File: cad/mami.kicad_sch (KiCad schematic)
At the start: 86 parts, among them SW1 SW_Push, SW10 SW_Push, SW11 SW_Push, SW12 SW_Push, SW13 SW_Push, SW14 SW_Push, SW15 SW_Push, SW16 SW_Push, SW17 SW_Push, SW18 SW_Push, SW19 SW_Push, SW2 SW_Push, SW20 SW_Push, SW21 SW_Push, SW22 SW_Push, SW23 SW_Push, SW24 SW_Push, SW25 SW_Push, SW26 SW_Push, SW27 SW_Push, SW28 SW_Push, SW29 SW_Push, SW3 SW_Push, SW30 SW_Push, SW31 SW_Push, SW32 SW_Push, SW33 SW_Push, SW34 SW_Push, SW35 SW_Push, SW36 SW_Push, SW37 SW_Push, SW38 SW_Push, SW39 SW_Push, SW4 SW_Push, SW40 SW_Push, SW41 SW_Push, SW42 SW_Push, SW43 ResetSW, SW5 SW_Push, SW6 SW_Push, SW7 SW_Push, SW8 SW_Push, SW9 SW_Push, U1 ProMicro

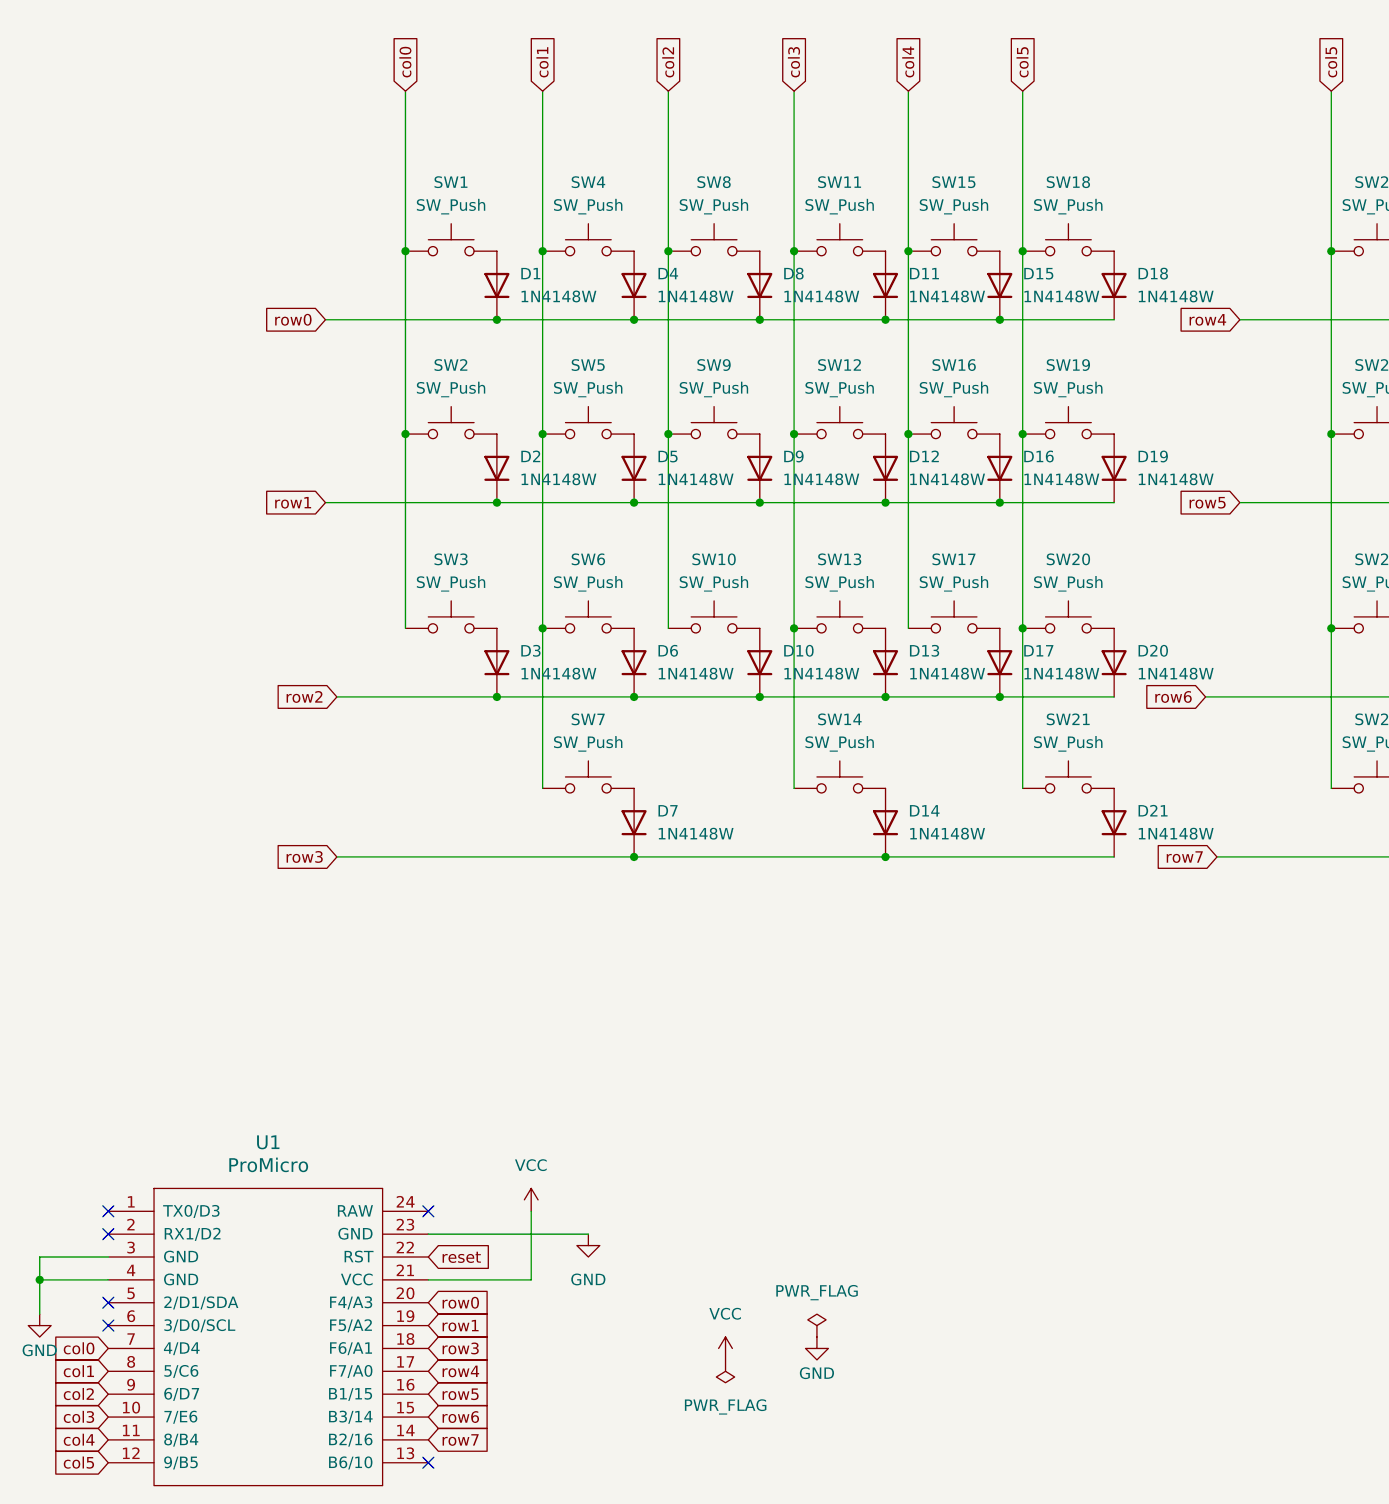
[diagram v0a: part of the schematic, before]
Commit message: symmetric schema update pcb
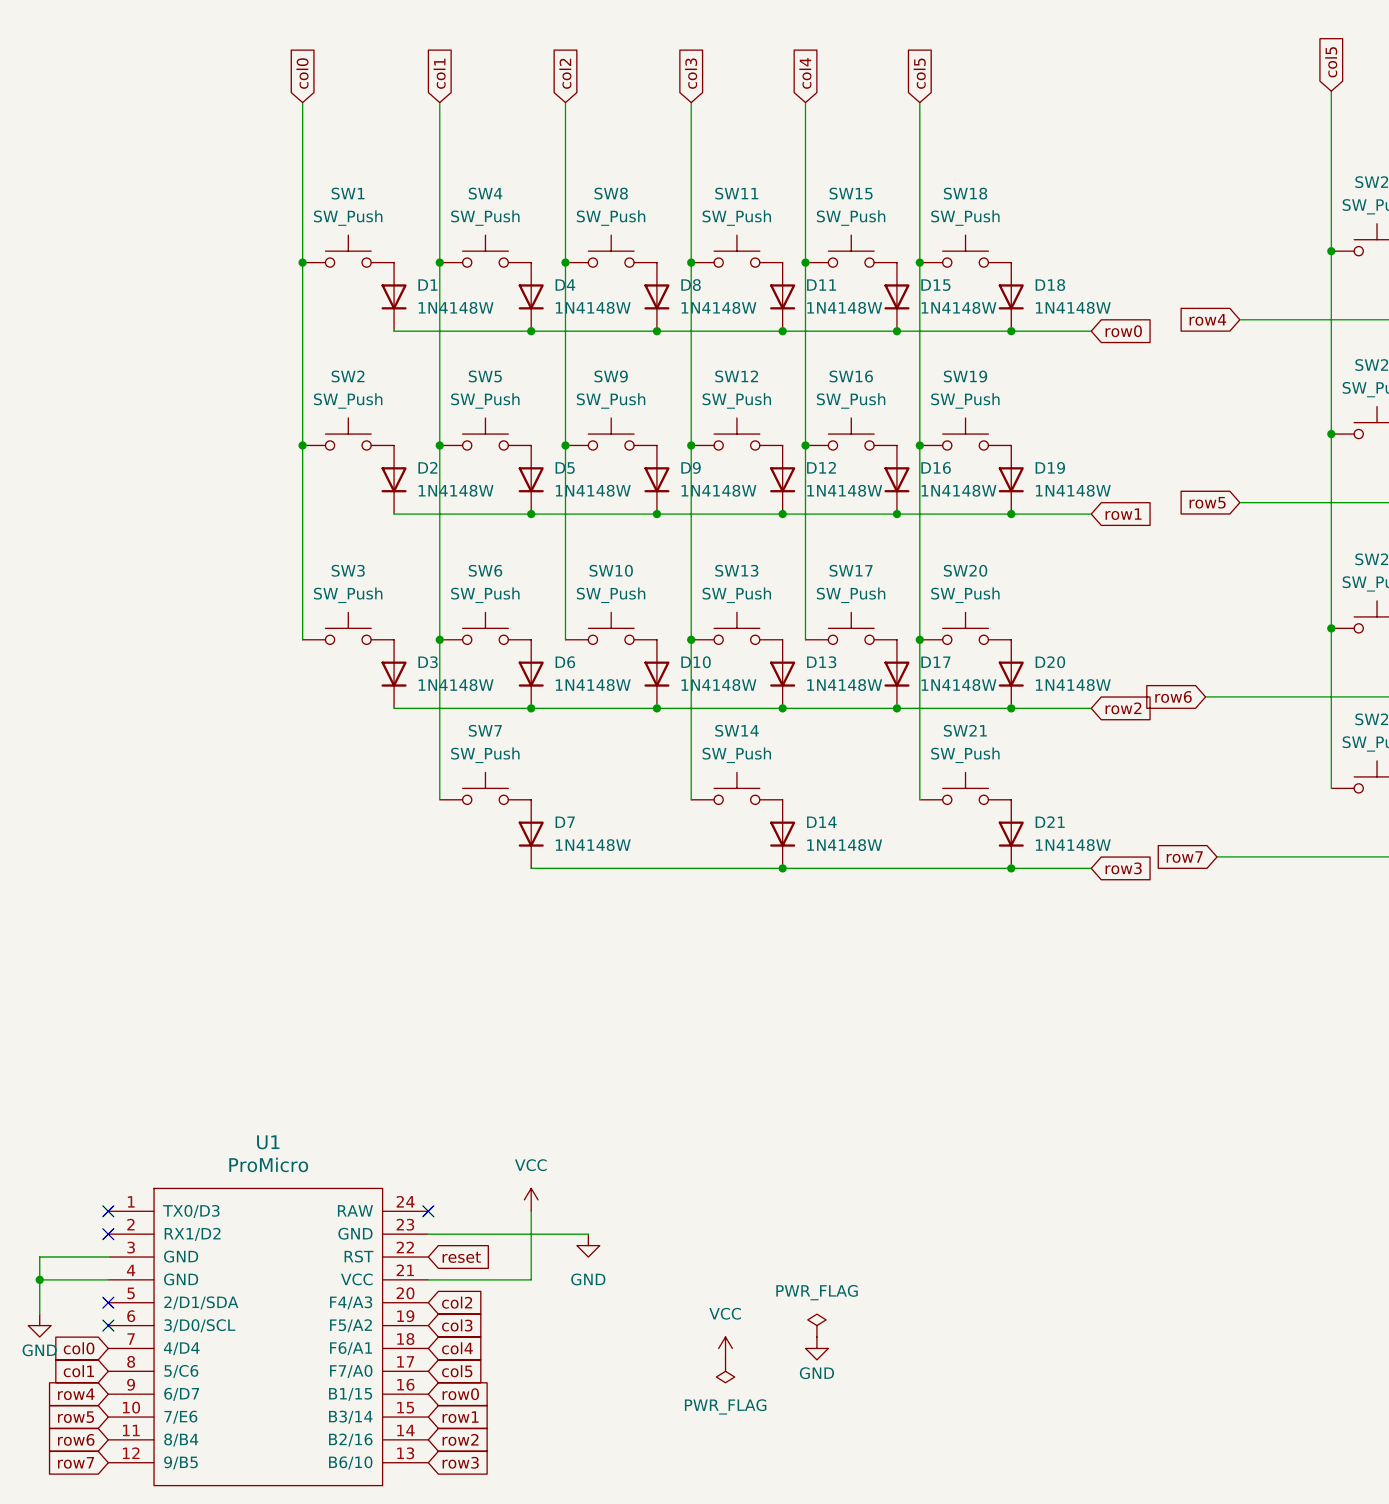
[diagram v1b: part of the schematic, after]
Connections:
- net col2: now also U1.20 (F4/A3); no longer U1.9 (6/D7)
- net col3: now also U1.19 (F5/A2); no longer U1.10 (7/E6)
- net col4: now also U1.18 (F6/A1); no longer U1.11 (8/B4)
- net col5: now also U1.17 (F7/A0); no longer U1.12 (9/B5)
- net row0: now also U1.16 (B1/15); no longer U1.20 (F4/A3)
- net row1: now also U1.15 (B3/14); no longer U1.19 (F5/A2)
- net row2: now also U1.14 (B2/16)
- net row3: now also U1.13 (B6/10); no longer U1.18 (F6/A1)
- net row4: now also U1.9 (6/D7); no longer U1.17 (F7/A0)
- net row5: now also U1.10 (7/E6); no longer U1.16 (B1/15)
- net row6: now also U1.11 (8/B4); no longer U1.15 (B3/14)
- net row7: now also U1.12 (9/B5); no longer U1.14 (B2/16)
- no-connect marks 6 -> 5
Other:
- moved on the sheet: D1, D10, D11, D12, D13, D14, D15, D16, D17, D18, D19, D2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

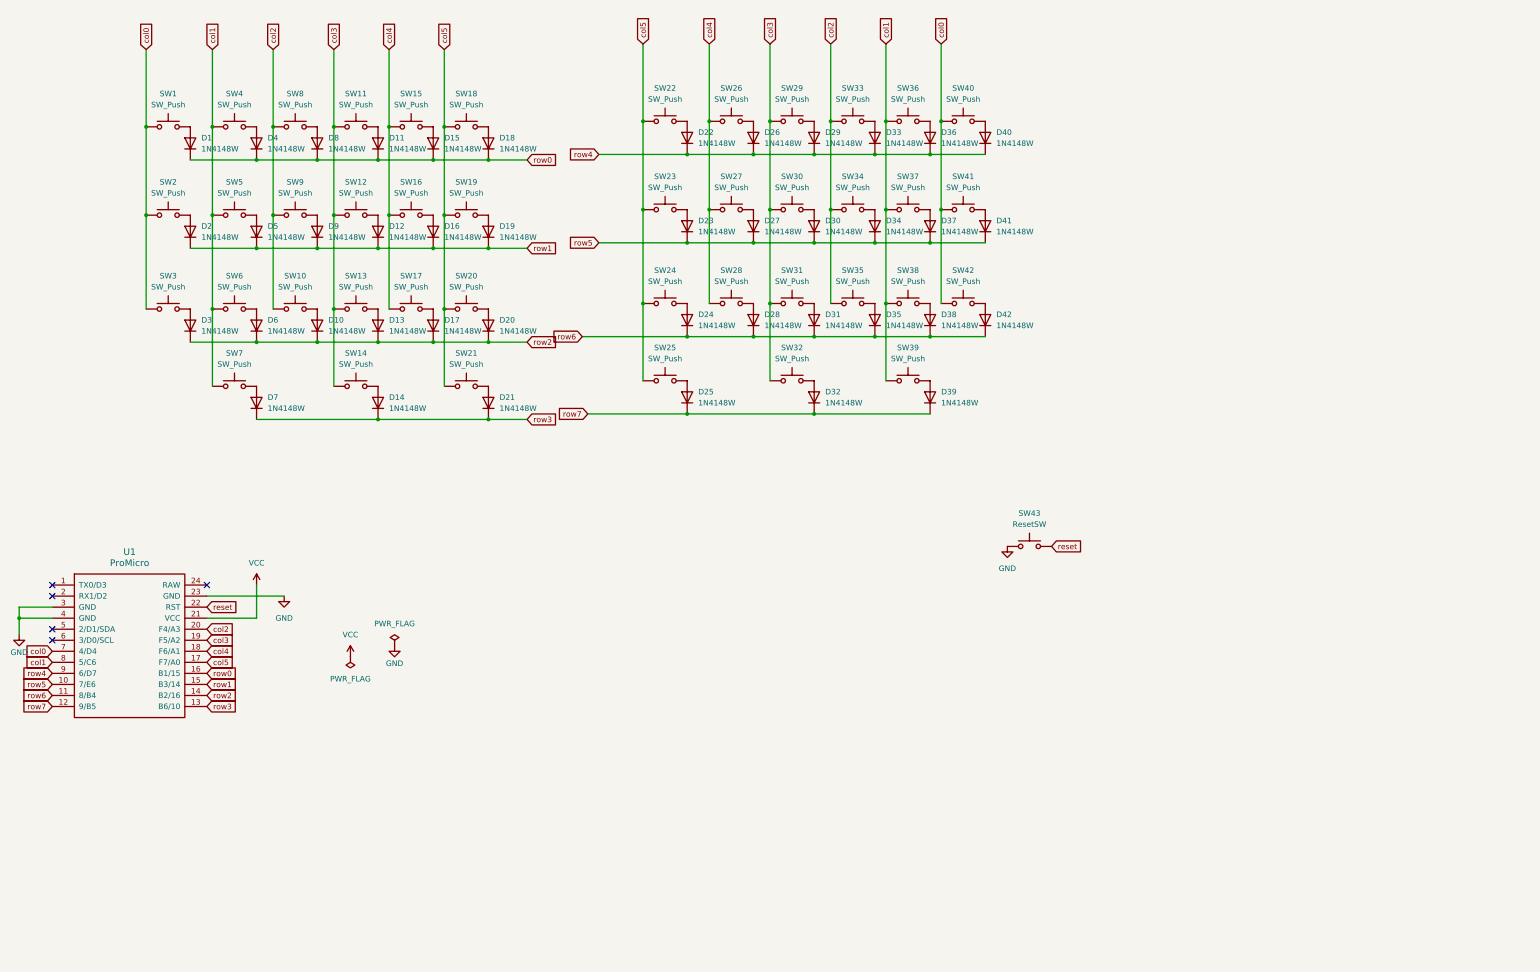
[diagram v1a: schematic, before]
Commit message: 回路図エディターをbattery有り＋LED有りに変更
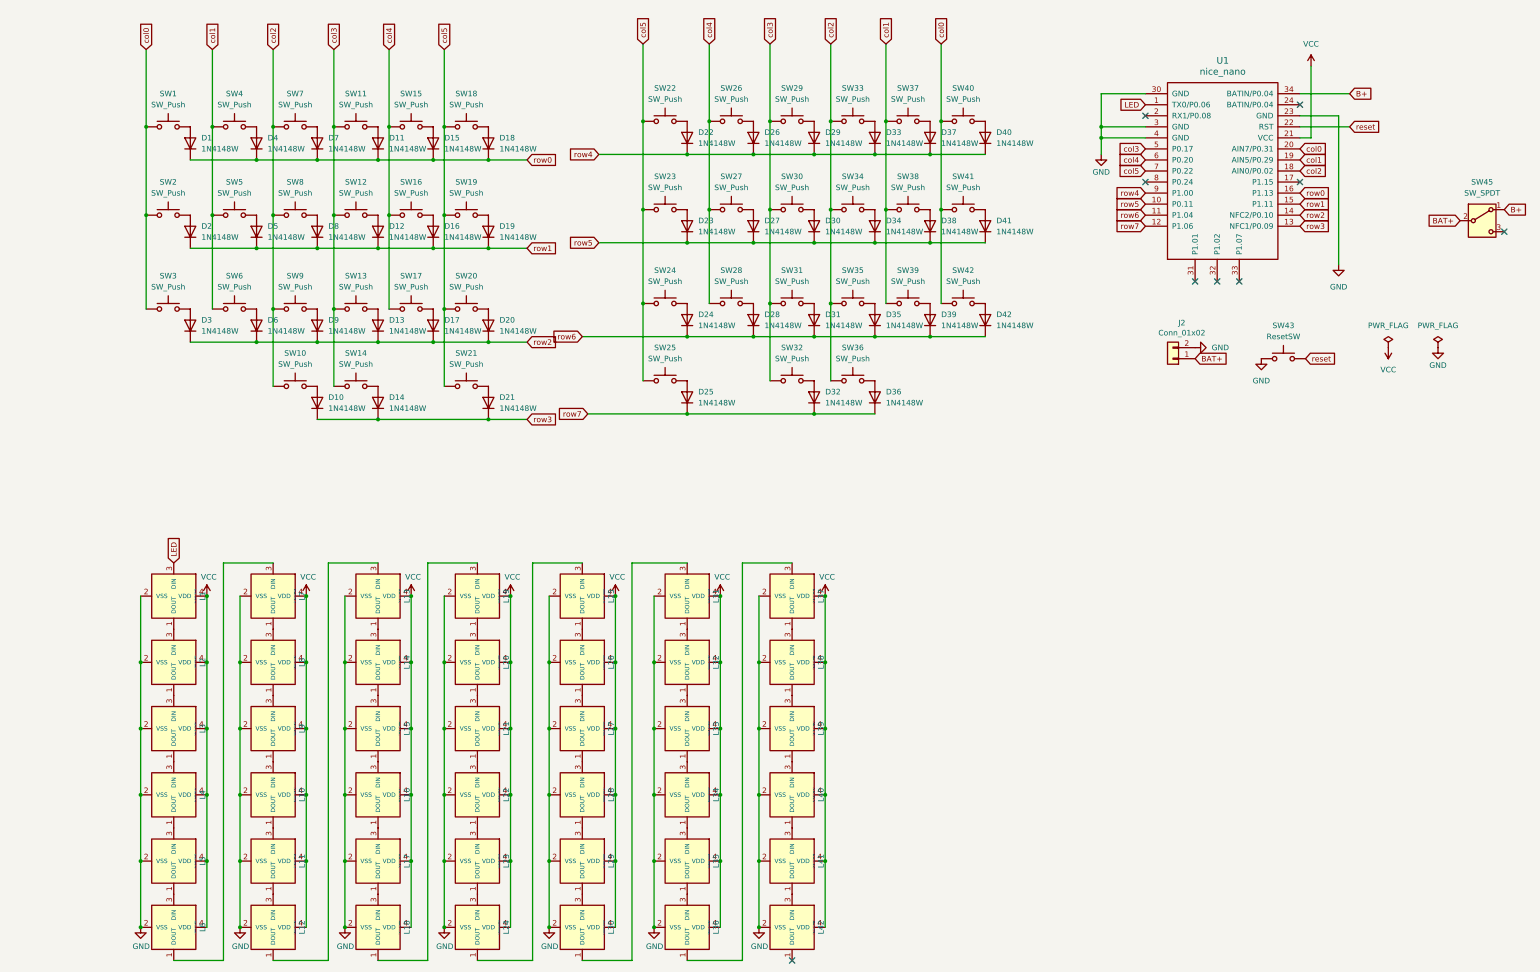
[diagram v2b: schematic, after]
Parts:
- removed U1: ProMicro, kbd:ProMicro, symbol kbd:ProMicro
- added J2: Conn_01x02, kbd_Parts:Battery_BMP_2pin, symbol Connector_Generic:Conn_01x02
- added L1, L10, L11, L12, L13, L14, L15, L16, L17, L18, L19, L2, L20, L21, L22, L23, L24, L25, L26, L27, L28, L29, L3, L30, L31, L32, L33, L34, L35, L36, L37, L38, L39, L4, L40, L41, L42, L5, L6, L7, L8, L9: SK6812MINI, kbd_Parts:LED_SK6812MINI-E_BL, symbol Salicylic_kbd:LED_SK6812MINI-E
- added SW45: SW_SPDT, symbol Switch:SW_SPDT
- added U1: nice_nano, symbol mylib:nice_nano
- renumbered D7 to D10, D39 to D36, D36 to D37, D37 to D38, D38 to D39, D8 to D7, D9 to D8, D10 to D9, SW7 to SW10, SW39 to SW36, SW36 to SW37, SW37 to SW38, SW38 to SW39, SW8 to SW7, SW9 to SW8, SW10 to SW9
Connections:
- net GND: now also J2.2 (Pin_2), L1.2 (VSS), L10.2 (VSS), L11.2 (VSS), L12.2 (VSS), L13.2 (VSS), L14.2 (VSS), L15.2 (VSS), L16.2 (VSS), L17.2 (VSS), L18.2 (VSS), L19.2 (VSS), L2.2 (VSS), L20.2 (VSS), L21.2 (VSS), L22.2 (VSS), L23.2 (VSS), L24.2 (VSS), L25.2 (VSS), L26.2 (VSS), L27.2 (VSS), L28.2 (VSS), L29.2 (VSS), L3.2 (VSS), L30.2 (VSS), L31.2 (VSS), L32.2 (VSS), L33.2 (VSS), L34.2 (VSS), L35.2 (VSS), L36.2 (VSS), L37.2 (VSS), L38.2 (VSS), L39.2 (VSS), L4.2 (VSS), L40.2 (VSS), L41.2 (VSS), L42.2 (VSS), L5.2 (VSS), L6.2 (VSS), L7.2 (VSS), L8.2 (VSS), L9.2 (VSS), U1.23 (GND), U1.3 (GND), U1.30 (GND), U1.4 (GND)
- net VCC: now also L1.4 (VDD), L10.4 (VDD), L11.4 (VDD), L12.4 (VDD), L13.4 (VDD), L14.4 (VDD), L15.4 (VDD), L16.4 (VDD), L17.4 (VDD), L18.4 (VDD), L19.4 (VDD), L2.4 (VDD), L20.4 (VDD), L21.4 (VDD), L22.4 (VDD), L23.4 (VDD), L24.4 (VDD), L25.4 (VDD), L26.4 (VDD), L27.4 (VDD), L28.4 (VDD), L29.4 (VDD), L3.4 (VDD), L30.4 (VDD), L31.4 (VDD), L32.4 (VDD), L33.4 (VDD), L34.4 (VDD), L35.4 (VDD), L36.4 (VDD), L37.4 (VDD), L38.4 (VDD), L39.4 (VDD), L4.4 (VDD), L40.4 (VDD), L41.4 (VDD), L42.4 (VDD), L5.4 (VDD), L6.4 (VDD), L7.4 (VDD), L8.4 (VDD), L9.4 (VDD), U1.21 (VCC)
- net col0: now also U1.20 (AIN7/P0.31)
- net col1: now also U1.19 (AIN5/P0.29); no longer SW10.1, SW36.1
- net col2: now also SW10.1, SW36.1, U1.18 (AIN0/P0.02)
- net col3: now also U1.5 (P0.17)
- net col4: now also U1.6 (P0.20)
- net col5: now also U1.7 (P0.22)
- net reset: now also U1.22 (RST)
- net row0: now also U1.16 (P1.13)
- net row1: now also U1.15 (P1.11)
- net row2: now also U1.14 (NFC2/P0.10)
- net row3: now also U1.13 (NFC1/P0.09)
- net row4: now also U1.9 (P1.00)
- net row5: now also U1.10 (P0.11)
- net row6: now also U1.11 (P1.04)
- net row7: now also U1.12 (P1.06)
- new net: L19.1 (DOUT), L20.3 (DIN)
- new net: L18.1 (DOUT), L19.3 (DIN)
- new net: L39.1 (DOUT), L40.3 (DIN)
- new net: L38.1 (DOUT), L39.3 (DIN)
- new net: L7.1 (DOUT), L8.3 (DIN)
- new net: L6.1 (DOUT), L7.3 (DIN)
- new net: L4.1 (DOUT), L5.3 (DIN)
- new net: L3.1 (DOUT), L4.3 (DIN)
- new net: L26.1 (DOUT), L27.3 (DIN)
- new net: L25.1 (DOUT), L26.3 (DIN)
- new net: L17.1 (DOUT), L18.3 (DIN)
- new net: L41.1 (DOUT), L42.3 (DIN)
- new net: L29.1 (DOUT), L30.3 (DIN)
- new net: L28.1 (DOUT), L29.3 (DIN)
- new net: L5.1 (DOUT), L6.3 (DIN)
- new net: L1.1 (DOUT), L2.3 (DIN)
- new net: L27.1 (DOUT), L28.3 (DIN)
- new net: L10.1 (DOUT), L11.3 (DIN)
- new net: L10.3 (DIN), L9.1 (DOUT)
- new net: L11.1 (DOUT), L12.3 (DIN)
- new net: L16.1 (DOUT), L17.3 (DIN)
- new net: L8.1 (DOUT), L9.3 (DIN)
- new net: L24.1 (DOUT), L25.3 (DIN)
- new net: L12.1 (DOUT), L13.3 (DIN)
- new net: L40.1 (DOUT), L41.3 (DIN)
- new net: L2.1 (DOUT), L3.3 (DIN)
- new net: L37.1 (DOUT), L38.3 (DIN)
- new net: L36.1 (DOUT), L37.3 (DIN)
- new net: L35.1 (DOUT), L36.3 (DIN)
- new net: L21.1 (DOUT), L22.3 (DIN)
- new net: L20.1 (DOUT), L21.3 (DIN)
- new net: L31.1 (DOUT), L32.3 (DIN)
- new net: L30.1 (DOUT), L31.3 (DIN)
- new net: L15.1 (DOUT), L16.3 (DIN)
- new net: L34.1 (DOUT), L35.3 (DIN)
- new net: L33.1 (DOUT), L34.3 (DIN)
- new net: L22.1 (DOUT), L23.3 (DIN)
- new net: L23.1 (DOUT), L24.3 (DIN)
- new net: L14.1 (DOUT), L15.3 (DIN)
- new net: L13.1 (DOUT), L14.3 (DIN)
- new net: L32.1 (DOUT), L33.3 (DIN)
- new net B+: SW45.1 (A), U1.34 (BATIN/P0.04)
- new net BAT+: J2.1 (Pin_1), SW45.2 (B)
- new net LED: L1.3 (DIN), U1.1 (TX0/P0.06)
- no-connect marks 5 -> 9
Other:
- moved on the sheet: D10, D36, SW10, SW36, SW43
